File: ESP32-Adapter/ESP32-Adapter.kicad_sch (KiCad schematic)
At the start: 17 parts, among them J10 Barrel_Jack, J12 Conn_01x05, J13 Conn_01x05, J2 Conn_01x03, J3 Conn_01x03, J5 Conn_01x03, U1 ESP32-C5-DevKitC-1, U2 LM317DCYR, U3 Adafruit CANPAL, U4 ADAFRUIT INA219 BREAKOUT

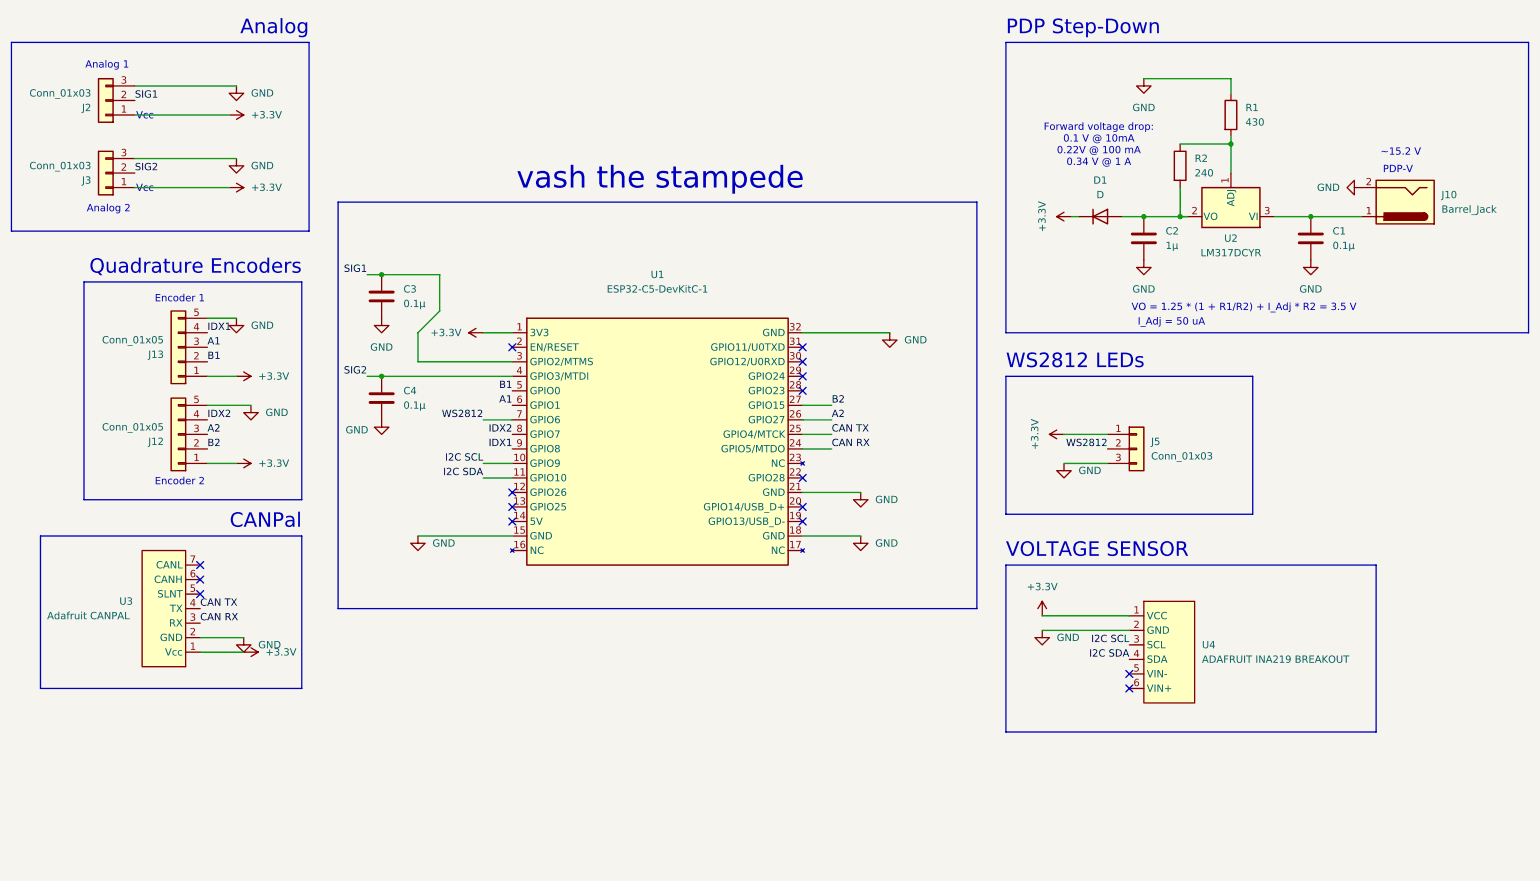
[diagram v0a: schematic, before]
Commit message: updates updates
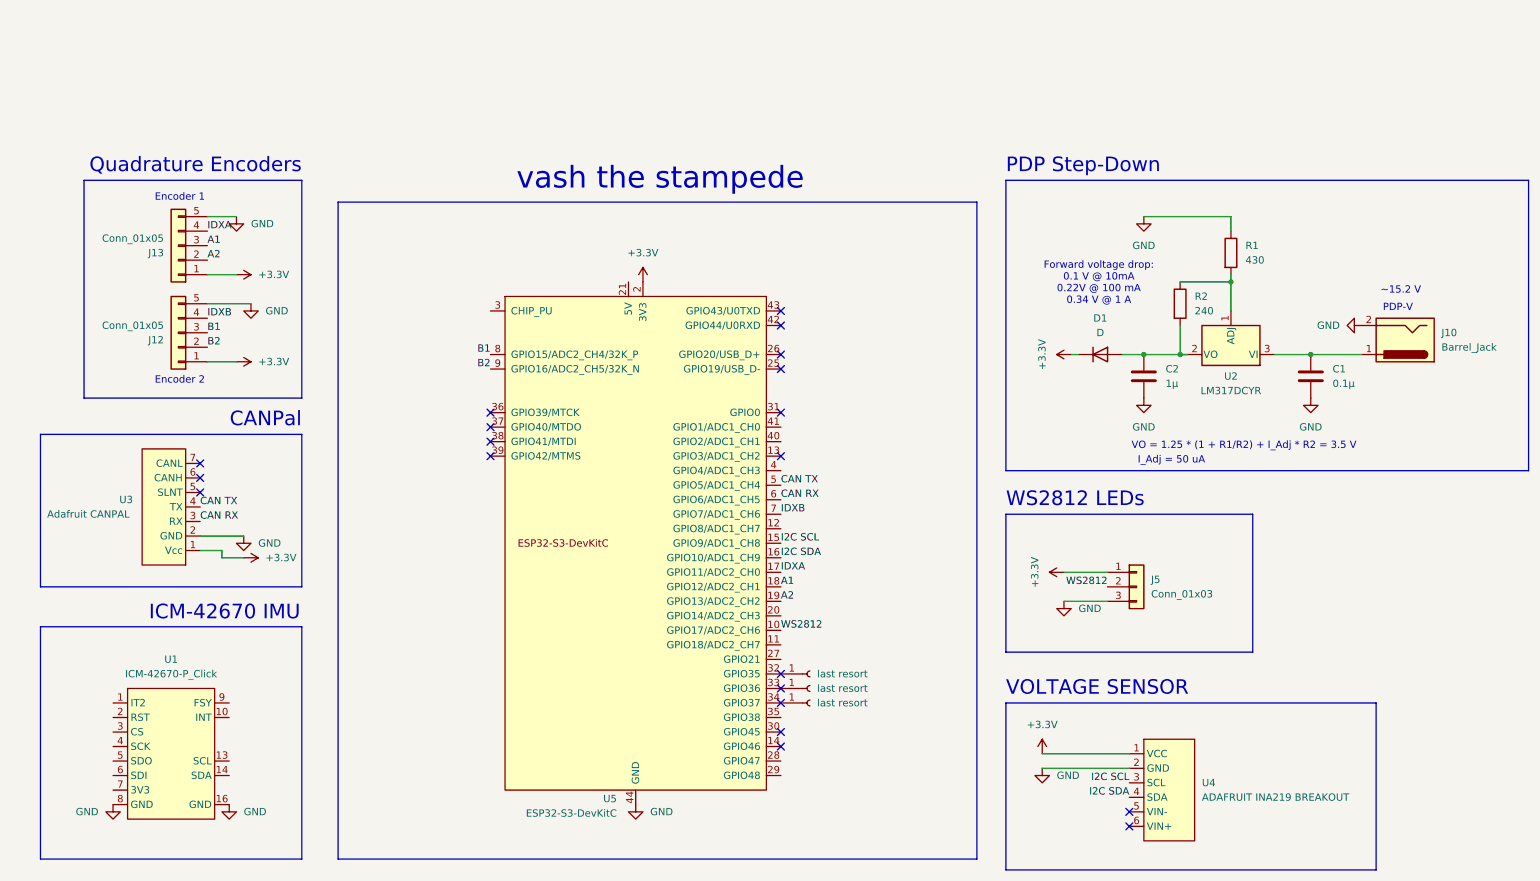
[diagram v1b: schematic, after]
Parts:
- removed C3, C4: 0.1µ, Capacitor_SMD:C_0402_1005Metric, symbol Device:C
- removed J2, J3: Conn_01x03, Connector_JST:JST_XH_S3B-XH-A-1_1x03_P2.50mm_Horizontal, symbol Connector_Generic:Conn_01x03
- removed U1: ESP32-C5-DevKitC-1, PCM_Espressif:ESP32-C5-DevKitC-1, symbol PCM_Espressif:ESP32-C5-DevKitC-1
- added J1, J2, J3: last resort, symbol Connector:Conn_01x01_Socket
- added U1: ICM-42670-P_Click, symbol Sensor_Motion:ICM-42670-P_Click
- added U5: ESP32-S3-DevKitC, PCM_Espressif:ESP32-S3-DevKitC, symbol PCM_Espressif:ESP32-S3-DevKitC
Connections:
- net +3.3V: now also U5.1 (3V3), U5.2 (3V3)
- net A1: now also U5.18 (GPIO12/ADC2_CH1)
- net A2: now also J13.2 (Pin_2), U5.19 (GPIO13/ADC2_CH2); no longer J12.3 (Pin_3)
- net B1: now also J12.3 (Pin_3), U5.8 (GPIO15/ADC2_CH4/32K_P); no longer J13.2 (Pin_2)
- net B2: now also U5.9 (GPIO16/ADC2_CH5/32K_N)
- net CAN RX: now also U5.6 (GPIO6/ADC1_CH5)
- net CAN TX: now also U5.5 (GPIO5/ADC1_CH4)
- net GND: now also U1.16 (GND), U1.8 (GND), U5.22 (GND), U5.23 (GND), U5.24 (GND), U5.44 (GND)
- net I2C SCL: now also U5.15 (GPIO9/ADC1_CH8)
- net I2C SDA: now also U5.16 (GPIO10/ADC1_CH9)
- net WS2812: now also U5.10 (GPIO17/ADC2_CH6)
- net IDX1 renamed IDXA
- net IDXA: now also U5.17 (GPIO11/ADC2_CH0)
- net IDX2 renamed IDXB
- net IDXB: now also U5.7 (GPIO7/ADC1_CH6)
- new net: J1.1 (Pin_1), U5.32 (GPIO35)
- new net: J2.1 (Pin_1), U5.33 (GPIO36)
- new net: J3.1 (Pin_1), U5.34 (GPIO37)
- no-connect marks 16 -> 20
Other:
- note added: "ICM-42670 IMU"
- note removed: "Analog"
- note removed: "Analog 1"
- note removed: "Analog 2"
- note removed: "Vcc"
- moved on the sheet: C1, C2, D1, J10, J12, J13, J5, R1, R2, U2, U3, U4
